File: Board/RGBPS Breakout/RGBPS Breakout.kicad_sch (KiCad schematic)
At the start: 4 parts, among them IC1 APDS-9999, J1 Conn_01x04_Pin

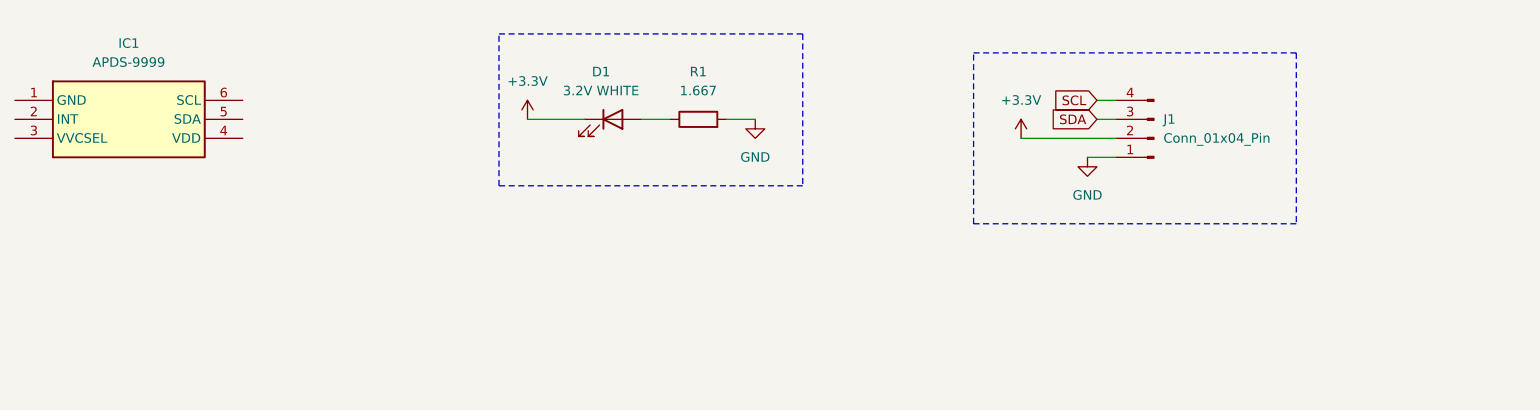
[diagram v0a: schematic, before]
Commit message: partially done with power
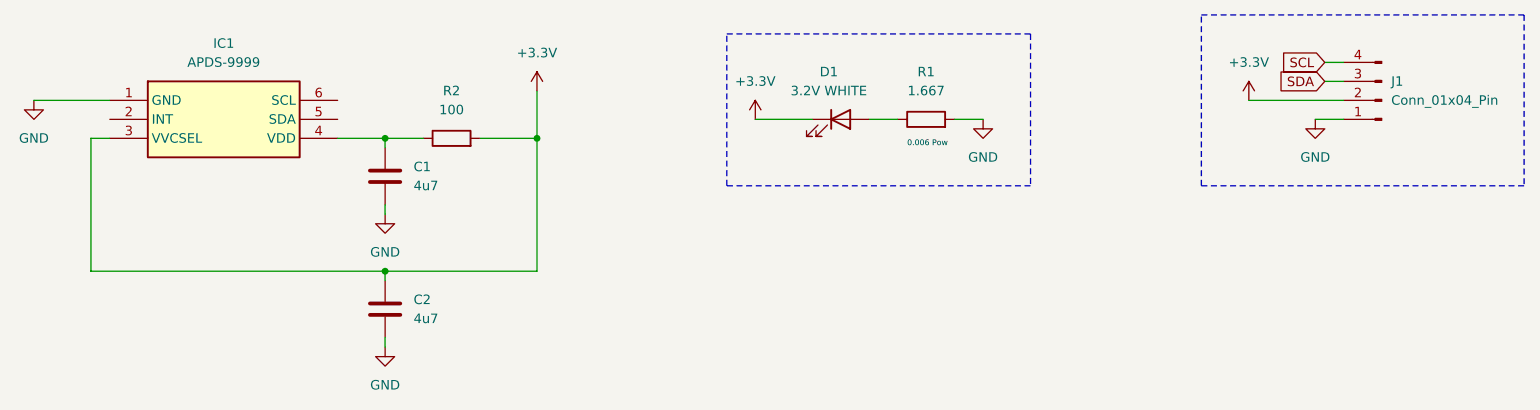
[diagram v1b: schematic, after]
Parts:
- added C1, C2: 4u7, symbol Device:C
- added R2: 100, symbol Device:R
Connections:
- net +3.3V: now also IC1.3 (VVCSEL), C2.1, R2.2
- net GND: now also IC1.1 (GND), C1.2, C2.2
- net at IC1.4 (VDD): now also C1.1, R2.1
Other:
- moved on the sheet: D1, IC1, J1, R1
